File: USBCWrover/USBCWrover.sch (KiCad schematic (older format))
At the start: 21 parts, among them J1 USB_C_Receptacle_USB2.0, Q1 Q_NMOS_GSD, Q2 Q_NMOS_GSD, SW1 SW_Push, SW2 SW_Push, U1 CH340C, U2 CP2104, U3 AMS1117-3.3

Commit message: routing done, but not pretty
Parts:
- removed C3: 100nF, Capacitor_SMD:C_0603_1608Metric, symbol Device:C
- removed Q1, Q2: Q_NMOS_GSD, Package_TO_SOT_SMD:SOT-23, symbol Device:Q_NMOS_GSD
- removed R3, R4: 10k, Resistor_SMD:R_0603_1608Metric, symbol Device:R
- removed SW2: SW_Push, Button_Switch_SMD:SW_Push_1P1T_NO_6x6mm_H9.5mm, symbol Switch:SW_Push
- removed U1: CH340C, Package_SO:SOIC-16_3.9x9.9mm_P1.27mm, symbol Interface_USB:CH340C
- added J2, J3: Conn_02x10_Odd_Even, Connector_PinHeader_2.54mm:PinHeader_2x10_P2.54mm_Vertical, symbol Connector_Generic:Conn_02x10_Odd_Even
- added U1: UMH3N, Package_SO:TSOP-6_1.65x3.05mm_P0.95mm, symbol UMH3N:UMH3N
- added U4: ESP32-WROVER, esp32-wrover:ESP32-WROVER, symbol esp32-wrover:ESP32-WROVER
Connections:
- net labels added: CLK_IO6, CMD_IO11, IO12, IO13, IO14, IO15, IO18, IO19, IO2, IO21, IO22, IO23, IO25, IO26, IO27, IO32, IO33, IO34, IO35, IO4, IO5, SD0_IO7, SD1_IO8, SD2_IO9, SD3_IO10, SENSOR_VN, Sensor_VP
- wire segments 77 -> 72

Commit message: lot prettier
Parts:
- removed U3: AMS1117-3.3, Package_TO_SOT_SMD:SOT-223-3_TabPin2, symbol Regulator_Linear:AMS1117-3.3
- added U3: HX9193-33GB, Package_TO_SOT_SMD:SOT-23-5, symbol Regulator_Linear:MIC5504-3.3YM5
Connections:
- net labels added: IO16, IO17
- wire segments 72 -> 75
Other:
- moved on the sheet: C4, C5, C6, C7
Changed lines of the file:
@@
-$EndComp
-$Comp
-L Regulator_Linear:AMS1117-3.3 U3
-U 1 1 5F42D349
-P 8500 5350
-F 0 "U3" H 8500 5592 50  0000 C CNN
-F 1 "AMS1117-3.3" H 8500 5501 50  0000 C CNN
-F 2 "Package_TO_SOT_SMD:SOT-223-3_TabPin2" H 8500 5550 50  0001 C CNN
-F 3 "http://www.advanced-monolithic.com/pdf/ds1117.pdf" H 8600 5100 50  0001 C CNN
-	1    8500 5350
-	1    0    0    -1
 $EndComp
 $Comp
 L power:+5V #PWR021
 U 1 1 5F42F75C
-P 7350 5300
-F 0 "#PWR021" H 7350 5150 50  0001 C CNN
-F 1 "+5V" H 7365 5473 50  0000 C CNN
-F 2 "" H 7350 5300 50  0001 C CNN
-F 3 "" H 7350 5300 50  0001 C CNN
-	1    7350 5300
+P 7000 4350
+F 0 "#PWR021" H 7000 4200 50  0001 C CNN
+F 1 "+5V" H 7015 4523 50  0000 C CNN
+F 2 "" H 7000 4350 50  0001 C CNN
+F 3 "" H 7000 4350 50  0001 C CNN
+	1    7000 4350
 	1    0    0    -1
 $EndComp
@@
 L power:+3.3V #PWR027
 U 1 1 5F430357
-P 9650 5350
-F 0 "#PWR027" H 9650 5200 50  0001 C CNN
-F 1 "+3.3V" H 9665 5523 50  0000 C CNN
-F 2 "" H 9650 5350 50  0001 C CNN
-F 3 "" H 9650 5350 50  0001 C CNN
-	1    9650 5350
+P 9800 4400
+F 0 "#PWR027" H 9800 4250 50  0001 C CNN
+F 1 "+3.3V" H 9815 4573 50  0000 C CNN
+F 2 "" H 9800 4400 50  0001 C CNN
+F 3 "" H 9800 4400 50  0001 C CNN
+	1    9800 4400
 	1    0    0    -1
 $EndComp
@@
 L power:GND #PWR024
 U 1 1 5F4309D7
-P 8500 5750
-F 0 "#PWR024" H 8500 5500 50  0001 C CNN
-F 1 "GND" H 8505 5577 50  0000 C CNN
-F 2 "" H 8500 5750 50  0001 C CNN
-F 3 "" H 8500 5750 50  0001 C CNN
-	1    8500 5750
+P 8500 4900
+F 0 "#PWR024" H 8500 4650 50  0001 C CNN
+F 1 "GND" H 8505 4727 50  0000 C CNN
+F 2 "" H 8500 4900 50  0001 C CNN
+F 3 "" H 8500 4900 50  0001 C CNN
+	1    8500 4900
 	1    0    0    -1
 $EndComp
@@
 L Device:C C5
 U 1 1 5F4311CF
-P 7900 5500
-F 0 "C5" H 8015 5546 50  0000 L CNN
-F 1 "100nF" H 8015 5455 50  0000 L CNN
-F 2 "Capacitor_SMD:C_0603_1608Metric" H 7938 5350 50  0001 C CNN
-F 3 "~" H 7900 5500 50  0001 C CNN
-	1    7900 5500
+P 7550 4550
+F 0 "C5" H 7665 4596 50  0000 L CNN
+F 1 "100nF" H 7665 4505 50  0000 L CNN
+F 2 "Capacitor_SMD:C_0603_1608Metric" H 7588 4400 50  0001 C CNN
+F 3 "~" H 7550 4550 50  0001 C CNN
+	1    7550 4550
 	1    0    0    -1
 $EndComp
@@
 L Device:C C4
 U 1 1 5F432724
-P 7500 5500
-F 0 "C4" H 7615 5546 50  0000 L CNN
-F 1 "4u7" H 7615 5455 50  0000 L CNN
-F 2 "Capacitor_SMD:C_0603_1608Metric" H 7538 5350 50  0001 C CNN
-F 3 "~" H 7500 5500 50  0001 C CNN
-	1    7500 5500
-	1    0    0    -1
-$EndComp
-Wire Wire Line
-	7350 5300 7350 5350
-Wire Wire Line
-	7350 5350 7500 5350
-Wire Wire Line
-	7500 5350 7900 5350
-Connection ~ 7500 5350
-Wire Wire Line
-	7900 5350 8200 5350
-Connection ~ 7900 5350
+P 7150 4550
+F 0 "C4" H 7265 4596 50  0000 L CNN
+F 1 "4u7" H 7265 4505 50  0000 L CNN
+F 2 "Capacitor_SMD:C_0603_1608Metric" H 7188 4400 50  0001 C CNN
+F 3 "~" H 7150 4550 50  0001 C CNN
+	1    7150 4550
+	1    0    0    -1
+$EndComp
+Wire Wire Line
+	7000 4350 7000 4400
+Wire Wire Line
+	7000 4400 7150 4400
+Wire Wire Line
+	7150 4400 7550 4400
+Connection ~ 7150 4400
 $Comp
 L Device:C C6
 U 1 1 5F436356
-P 8950 5500
-F 0 "C6" H 9065 5546 50  0000 L CNN
-F 1 "100nF" H 9065 5455 50  0000 L CNN
-F 2 "Capacitor_SMD:C_0603_1608Metric" H 8988 5350 50  0001 C CNN
-F 3 "~" H 8950 5500 50  0001 C CNN
-	1    8950 5500
+P 9100 4550
+F 0 "C6" H 9215 4596 50  0000 L CNN
+F 1 "100nF" H 9215 4505 50  0000 L CNN
+F 2 "Capacitor_SMD:C_0603_1608Metric" H 9138 4400 50  0001 C CNN
+F 3 "~" H 9100 4550 50  0001 C CNN
+	1    9100 4550
 	1    0    0    -1
 $EndComp
@@
 L Device:C C7
 U 1 1 5F4367F1
-P 9450 5500
-F 0 "C7" H 9565 5546 50  0000 L CNN
-F 1 "4u7" H 9565 5455 50  0000 L CNN
-F 2 "Capacitor_SMD:C_0603_1608Metric" H 9488 5350 50  0001 C CNN
-F 3 "~" H 9450 5500 50  0001 C CNN
-	1    9450 5500
-	1    0    0    -1
-$EndComp
-Wire Wire Line
-	8800 5350 8950 5350
-Wire Wire Line
-	8950 5350 9450 5350
-Connection ~ 8950 5350
-Wire Wire Line
-	9650 5350 9450 5350
-Connection ~ 9450 5350
+P 9600 4550
+F 0 "C7" H 9715 4596 50  0000 L CNN
+F 1 "4u7" H 9715 4505 50  0000 L CNN
+F 2 "Capacitor_SMD:C_0603_1608Metric" H 9638 4400 50  0001 C CNN
+F 3 "~" H 9600 4550 50  0001 C CNN
+	1    9600 4550
+	1    0    0    -1
+$EndComp
+Wire Wire Line
+	9100 4400 9600 4400
+Wire Wire Line
+	9800 4400 9600 4400
+Connection ~ 9600 4400
 $Comp
 L power:GND #PWR022
 U 1 1 5F439A51
-P 7500 5750
-F 0 "#PWR022" H 7500 5500 50  0001 C CNN
-F 1 "GND" H 7505 5577 50  0000 C CNN
-F 2 "" H 7500 5750 50  0001 C CNN
-F 3 "" H 7500 5750 50  0001 C CNN
-	1    7500 5750
+P 7150 4800
+F 0 "#PWR022" H 7150 4550 50  0001 C CNN
+F 1 "GND" H 7155 4627 50  0000 C CNN
+F 2 "" H 7150 4800 50  0001 C CNN
+F 3 "" H 7150 4800 50  0001 C CNN
+	1    7150 4800
 	1    0    0    -1
 $EndComp
@@
 L power:GND #PWR023
 U 1 1 5F439DED
-P 7900 5750
-F 0 "#PWR023" H 7900 5500 50  0001 C CNN
-F 1 "GND" H 7905 5577 50  0000 C CNN
-F 2 "" H 7900 5750 50  0001 C CNN
-F 3 "" H 7900 5750 50  0001 C CNN
-	1    7900 5750
+P 7550 4800
+F 0 "#PWR023" H 7550 4550 50  0001 C CNN
+F 1 "GND" H 7555 4627 50  0000 C CNN
+F 2 "" H 7550 4800 50  0001 C CNN
+F 3 "" H 7550 4800 50  0001 C CNN
+	1    7550 4800
 	1    0    0    -1
 $EndComp
@@
 L power:GND #PWR025
 U 1 1 5F43A057
-P 8950 5750
-F 0 "#PWR025" H 8950 5500 50  0001 C CNN
-F 1 "GND" H 8955 5577 50  0000 C CNN
-F 2 "" H 8950 5750 50  0001 C CNN
-F 3 "" H 8950 5750 50  0001 C CNN
-	1    8950 5750
+P 9100 4800
+F 0 "#PWR025" H 9100 4550 50  0001 C CNN
+F 1 "GND" H 9105 4627 50  0000 C CNN
+F 2 "" H 9100 4800 50  0001 C CNN
+F 3 "" H 9100 4800 50  0001 C CNN
+	1    9100 4800
 	1    0    0    -1
 $EndComp
@@
 L power:GND #PWR026
 U 1 1 5F43A39E
-P 9450 5750
-F 0 "#PWR026" H 9450 5500 50  0001 C CNN
-F 1 "GND" H 9455 5577 50  0000 C CNN
-F 2 "" H 9450 5750 50  0001 C CNN
-F 3 "" H 9450 5750 50  0001 C CNN
-	1    9450 5750
-	1    0    0    -1
-$EndComp
-Wire Wire Line
-	8500 5750 8500 5650
-Wire Wire Line
-	7900 5750 7900 5650
-Wire Wire Line
-	7500 5750 7500 5650
-Wire Wire Line
-	8950 5750 8950 5650
-Wire Wire Line
-	9450 5650 9450 5750
+P 9600 4800
+F 0 "#PWR026" H 9600 4550 50  0001 C CNN
+F 1 "GND" H 9605 4627 50  0000 C CNN
+F 2 "" H 9600 4800 50  0001 C CNN
+F 3 "" H 9600 4800 50  0001 C CNN
+	1    9600 4800
+	1    0    0    -1
+$EndComp
+Wire Wire Line
+	7550 4800 7550 4700
+Wire Wire Line
+	7150 4800 7150 4700
+Wire Wire Line
+	9100 4800 9100 4700
+Wire Wire Line
+	9600 4700 9600 4800
 $Comp
 L power:+5V #PWR07
@@
 Text GLabel 5500 2650 0    50   Input ~ 0
 CLK_IO6
+Text GLabel 10300 2300 2    50   Input ~ 0
+IO17
+Text GLabel 10300 2400 2    50   Input ~ 0
+IO16
+Text GLabel 6000 2150 2    50   Input ~ 0
+IO17
+Text GLabel 6000 2250 2    50   Input ~ 0
+IO16
+$Comp
+L Regulator_Linear:MIC5504-3.3YM5 U3
+U 1 1 5F3EB1C6
+P 8500 4500
+F 0 "U3" H 8500 4867 50  0000 C CNN
+F 1 "HX9193-33GB" H 8500 4776 50  0000 C CNN
+F 2 "Package_TO_SOT_SMD:SOT-23-5" H 8500 4100 50  0001 C CNN
+F 3 "http://ww1.microchip.com/downloads/en/DeviceDoc/MIC550X.pdf" H 8250 4750 50  0001 C CNN
+	1    8500 4500
+	1    0    0    -1
+$EndComp
+Wire Wire Line
+	7550 4400 7950 4400
+Connection ~ 7550 4400
+Wire Wire Line
+	8100 4600 7950 4600
+Wire Wire Line
+	7950 4600 7950 4400
+Connection ~ 7950 4400
+Wire Wire Line
+	7950 4400 8100 4400
+Wire Wire Line
+	8900 4400 9100 4400
+Connection ~ 9100 4400
+Wire Wire Line
+	8500 4800 8500 4900
 $EndSCHEMATC

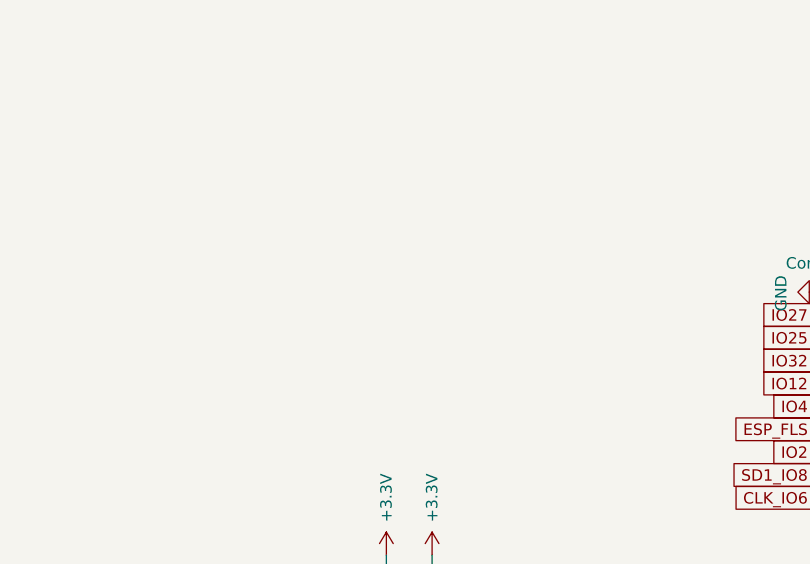
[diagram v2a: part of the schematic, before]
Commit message: now with art
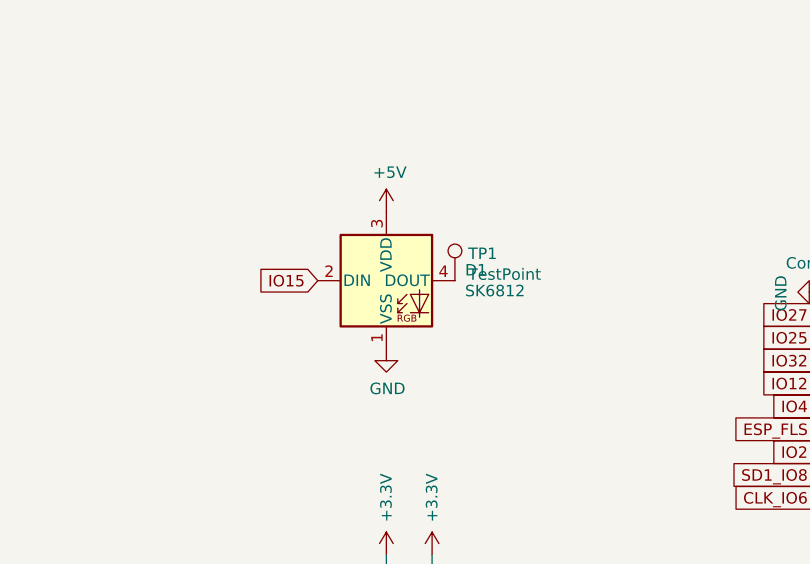
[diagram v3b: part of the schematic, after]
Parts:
- added D1: SK6812, LED_SMD:LED_SK6812_PLCC4_5.0x5.0mm_P3.2mm, symbol LED:SK6812
- added TP1: TestPoint, TestPoint:TestPoint_Pad_2.0x2.0mm, symbol Connector:TestPoint
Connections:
- net +5V: now also D1.3 (VDD)
- net GND: now also D1.1 (VSS)
- net IO15: now also D1.2 (DIN)
- new net: D1.4 (DOUT), TP1.1
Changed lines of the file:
@@
 Wire Wire Line
 	8500 4800 8500 4900
+$Comp
+L LED:SK6812 D1
+U 1 1 5F3F3DD8
+P 3600 1700
+F 0 "D1" H 3944 1746 50  0000 L CNN
+F 1 "SK6812" H 3944 1655 50  0000 L CNN
+F 2 "LED_SMD:LED_SK6812_PLCC4_5.0x5.0mm_P3.2mm" H 3650 1400 50  0001 L TNN
+F 3 "https://cdn-shop.adafruit.com/product-files/1138/SK6812+LED+datasheet+.pdf" H 3700 1325 50  0001 L TNN
+	1    3600 1700
+	1    0    0    -1
+$EndComp
+$Comp
+L power:+5V #PWR018
+U 1 1 5F3F4B3A
+P 3600 1400
+F 0 "#PWR018" H 3600 1250 50  0001 C CNN
+F 1 "+5V" H 3615 1573 50  0000 C CNN
+F 2 "" H 3600 1400 50  0001 C CNN
+F 3 "" H 3600 1400 50  0001 C CNN
+	1    3600 1400
+	1    0    0    -1
+$EndComp
+$Comp
+L power:GND #PWR028
+U 1 1 5F3F589D
+P 3600 2000
+F 0 "#PWR028" H 3600 1750 50  0001 C CNN
+F 1 "GND" H 3605 1827 50  0000 C CNN
+F 2 "" H 3600 2000 50  0001 C CNN
+F 3 "" H 3600 2000 50  0001 C CNN
+	1    3600 2000
+	1    0    0    -1
+$EndComp
+Text GLabel 3300 1700 0    50   Input ~ 0
+IO15
+$Comp
+L Connector:TestPoint TP1
+U 1 1 5F3FFC2D
+P 3900 1700
+F 0 "TP1" H 3958 1818 50  0000 L CNN
+F 1 "TestPoint" H 3958 1727 50  0000 L CNN
+F 2 "TestPoint:TestPoint_Pad_2.0x2.0mm" H 4100 1700 50  0001 C CNN
+F 3 "~" H 4100 1700 50  0001 C CNN
+	1    3900 1700
+	1    0    0    -1
+$EndComp
 $EndSCHEMATC

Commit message: rework
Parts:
- removed C1: 100nF, Capacitor_SMD:C_0603_1608Metric, symbol Device:C
- removed C2: 4.7uF, Capacitor_SMD:C_0603_1608Metric, symbol Device:C
- removed R1, R2: 5.1k, Resistor_SMD:R_0603_1608Metric, symbol Device:R
- removed R5, R6: 10k, Resistor_SMD:R_0603_1608Metric, symbol Device:R
- removed SW1: SW_Push, Button_Switch_SMD:SW_Push_1P1T_NO_6x6mm_H9.5mm, symbol Switch:SW_Push
- removed U2: CP2104, Package_DFN_QFN:QFN-24-1EP_4x4mm_P0.5mm_EP2.6x2.6mm, symbol Interface_USB:CP2104
- added D2: b5819w, Diode_SMD:D_SOD-123, symbol Device:D_Schottky
- added RN1: R_Pack04, Resistor_SMD:R_Array_Concave_4x0603, symbol Device:R_Pack04
- added SW2: SW_Push, Button_Switch_SMD:SW_Push_1P1T_NO_CK_KSC6xxJ, symbol Switch:SW_Push
- added U2: CH340C, Package_SO:SOIC-16_3.9x9.9mm_P1.27mm, symbol Interface_USB:CH340C
- C4, C5, C6, C7: footprint Capacitor_SMD:C_0603_1608Metric -> Capacitor_SMD:C_0805_2012Metric
- J2, J3: footprint Connector_PinHeader_2.54mm:PinHeader_2x10_P2.54mm_Vertical -> Connector_PinHeader_2.54mm:PinHeader_2x09_P2.54mm_Vertical; symbol Connector_Generic:Conn_02x10_Odd_Even -> Connector_Generic:Conn_02x09_Odd_Even
- TP1: footprint TestPoint:TestPoint_Pad_2.0x2.0mm -> TestPoint:TestPoint_Pad_1.0x1.0mm
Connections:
- net +3V3: now also RN1.1 (R1.1), RN1.2 (R2.1), U2.16 (VCC), U2.4 (V3)
- net +5V: now also D2.1 (K); no longer J1.A4 (VBUS), J1.A9 (VBUS), J1.B4 (VBUS), J1.B9 (VBUS)
- net ESP_FLS: now also RN1.7 (R2.2)
- net ESP_RST: now also RN1.8 (R1.2), SW2.1
- net ESP_RXD: now also U2.2 (TXD)
- net ESP_TXD: now also U2.3 (RXD)
- net GND: now also RN1.5 (R4.2), RN1.6 (R3.2), SW2.2, U2.1 (GND)
- net SER_DTR: now also U2.13 (~DTR)
- net SER_RTS: now also U2.14 (~RTS)
- net USB_D+: now also U2.5 (UD+)
- net USB_D-: now also U2.6 (UD-)
- net CC1: now reaches J1.A5 (CC1)
- net CC1: now also RN1.4 (R4.1)
- net CC2: now reaches J1.B5 (CC2)
- net CC2: now also RN1.3 (R3.1)
- net CLK_IO6: no longer names the net of U4.20 (CLK_IO6)
- net CLK_IO6: no longer J2.19 (Pin_19)
- net CMD_IO11: no longer names the net of U4.19 (CMD_IO11)
- net CMD_IO11: no longer J3.20 (Pin_20)
- net IO16: no longer names the net of U4.27 (IO16)
- net IO16: no longer J2.12 (Pin_12)
- net IO17: no longer names the net of U4.28 (IO17)
- net IO17: no longer J2.10 (Pin_10)
- net SD0_IO7: no longer names the net of U4.21 (SD0_IO7)
- net SD0_IO7: no longer J2.20 (Pin_20)
- net SD1_IO8: no longer names the net of U4.22 (SD1_IO8)
- net SD1_IO8: no longer J2.17 (Pin_17)
- net SD2_IO9: no longer names the net of U4.17 (SD2_IO9)
- net SD2_IO9: no longer J3.18 (Pin_18)
- net SD3_IO10: no longer names the net of U4.18 (SD3_IO10)
- net SD3_IO10: no longer J3.19 (Pin_19)
- new net VUSB: D2.2 (A), J1.A4 (VBUS), J1.A9 (VBUS), J1.B4 (VBUS), J1.B9 (VBUS)
- no-connect marks 0 -> 6
